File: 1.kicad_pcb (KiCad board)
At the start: 2 copper layers, 60 parts, among them J1 ValveOUT, J10 ResOUT, J2 220V_IN, J3 MotorOUT, J4 PumpOUT, J5 ISCP, J6 ButtonOUT, J7 SwitchOUT, J8 FloatOUT, J9 LedOUT, Q1 BT136, Q2 BT136, Q3 BT136, SW1 SW_Push, U1 ATmega8A-AU, U2 MOC3023M, U3 MOC3023M, U4 MOC3023M, Y1 16MHz

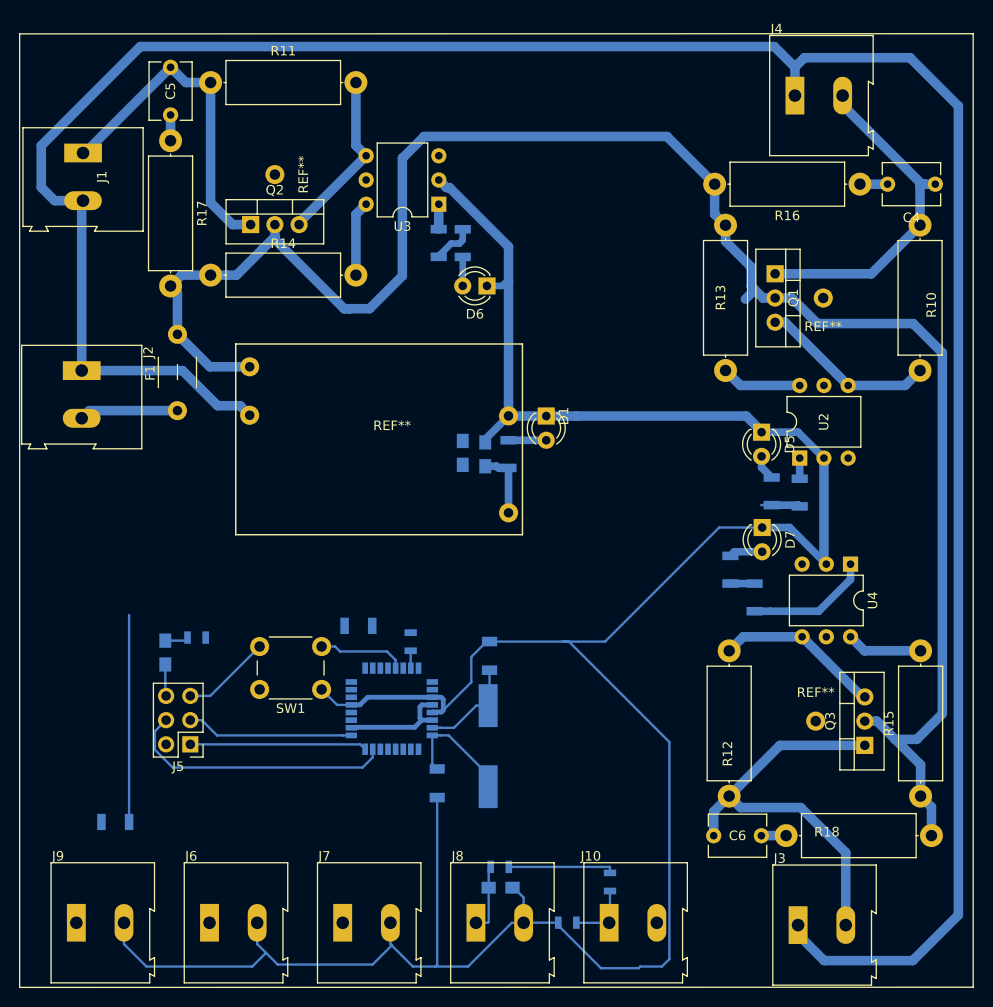
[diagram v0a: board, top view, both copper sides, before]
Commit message: 5.0
Плата готова
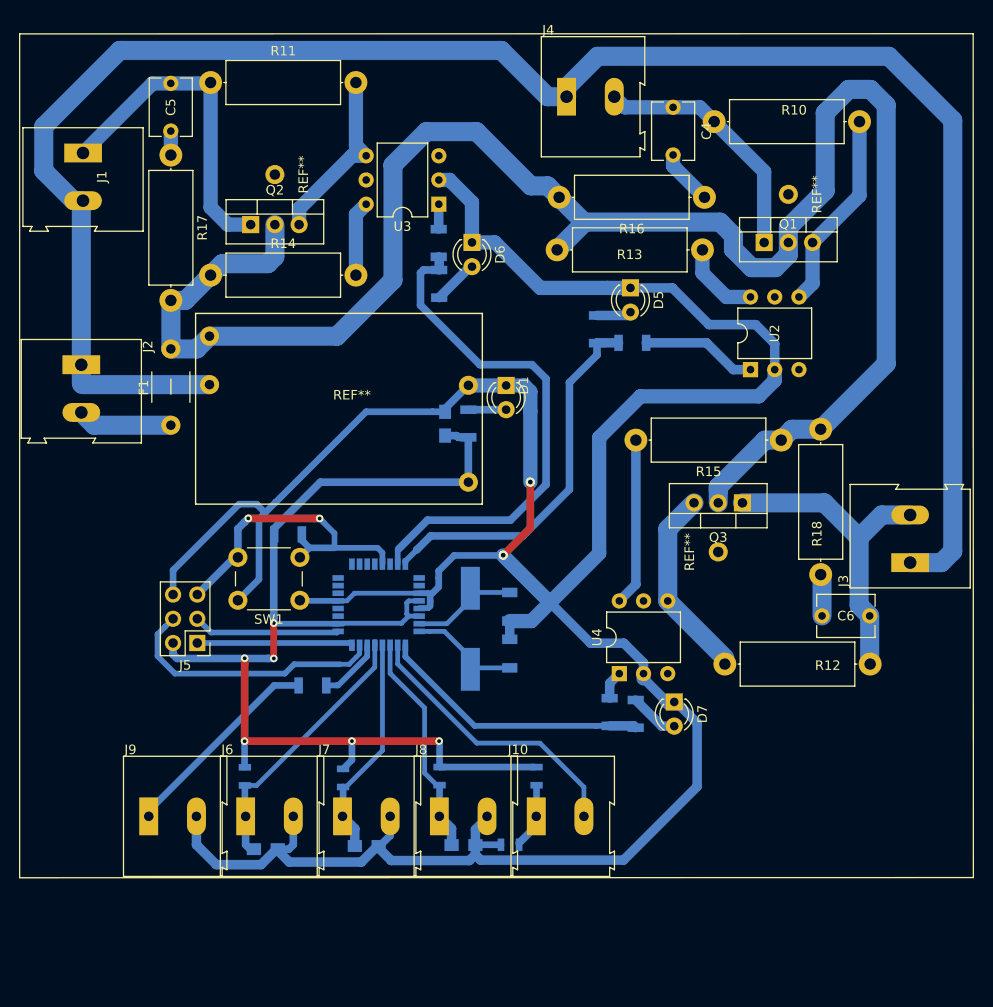
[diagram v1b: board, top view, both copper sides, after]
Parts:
- removed the REF** at (96.3, 39.7)
- removed the REF** at (95.5, 84.1)
- added REF**: , Measurement_Points:Measurement_Point_Round-TH_Big, F.Cu at (92.6, 28.8)
- added REF**: , Measurement_Points:Measurement_Point_Round-TH_Big, F.Cu at (85.3, 66.3)
- J10: value ResOUT -> PD6
- moved C8 42.4 mm to (48.4, 97.2), turned to 0 degrees
- moved R15 40.1 mm to (91.9, 54.6), turned to 180 degrees
- moved J3 39.8 mm to (105.4, 67.5), turned to 90 degrees
- moved C4 28.7 mm to (80.5, 19.7), turned to 270 degrees
- moved Q3 28.5 mm to (87.8, 61.2), turned to 180 degrees
- moved C6 28.3 mm to (101.2, 73.0), turned to 180 degrees
- moved R18 27.6 mm to (96.0, 68.7), turned to 90 degrees
- moved U4 26.8 mm to (74.9, 79.1), turned to 90 degrees
- moved R2 25.2 mm to (42.7, 80.3)
- moved R22 25.0 mm to (72.6, 43.0)
- moved R10 24.2 mm to (84.8, 21.2), turned to 0 degrees
- moved J4 24.0 mm to (69.4, 18.6)
- moved R6 23.5 mm to (76.3, 44.4), turned to 180 degrees
- moved C7 23.2 mm to (37.8, 97.5), turned to 0 degrees
- moved D7 20.5 mm to (80.7, 82.1)
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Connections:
- J10 pad 2: /PD5 -> /PD6
- U1 pad 10: Net-(U1-Pad10) -> /PD6
- U1 pad 11: Net-(U1-Pad11) -> /Float
- U1 pad 12: /PumpPin -> /Switch
- U1 pad 13: /ValvePin -> /Button
- U1 pad 14: /MotorPin -> Net-(R2-Pad2)
- U1 pad 2: Net-(R2-Pad2) -> Net-(U1-Pad2)
- U1 pad 30: /Button -> Net-(U1-Pad30)
- U1 pad 31: /Switch -> /ValvePin
- U1 pad 32: /Float -> /PumpPin
- U1 pad 9: /PD5 -> /MotorPin
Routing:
- net +5V: track 30.1 -> 121.5 mm, vias 0 -> 6
- net /220_In2: track 261.2 -> 199.6 mm
- net /ValvePin: track 4.44 -> 54.2 mm
- net /PumpPin: track 4.09 -> 39.4 mm
- net /PD6: track 0.00 -> 29.9 mm
- net Earth: track 285.2 -> 315.1 mm, vias 0 -> 2
- net /Button: track 2.46 -> 28.8 mm
- net /MotorPin: track 2.54 -> 28.4 mm
- net /Led: track 0.00 -> 21.7 mm
- net /Switch: track 1.84 -> 23.5 mm
- net /Float: track 7.23 -> 23.8 mm
- net /RST: track 18.6 -> 33.9 mm, vias 0 -> 2
- net Net-(R2-Pad2): track 21.7 -> 6.72 mm
- net Net-(R8-Pad1): track 13.0 -> 3.00 mm
- net Net-(R6-Pad1): track 2.16 -> 12.1 mm
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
